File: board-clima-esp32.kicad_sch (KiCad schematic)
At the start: 54 parts, among them IC1 ESP32-S3-WROOM-1-N4, J1 Conn_01x06_Pin, J2 Screw_Terminal_01x03, J3 Conn_01x04_Pin, J5 Conn_01x05_Pin, J6 USB_C_Receptacle, Q1 AO3400A, Q2 AO3401A, Q3 AO3400A, SW1 RESET, SW2 BOOT, U1 AMS1117-3.3, U3 PC817, U4 PC817

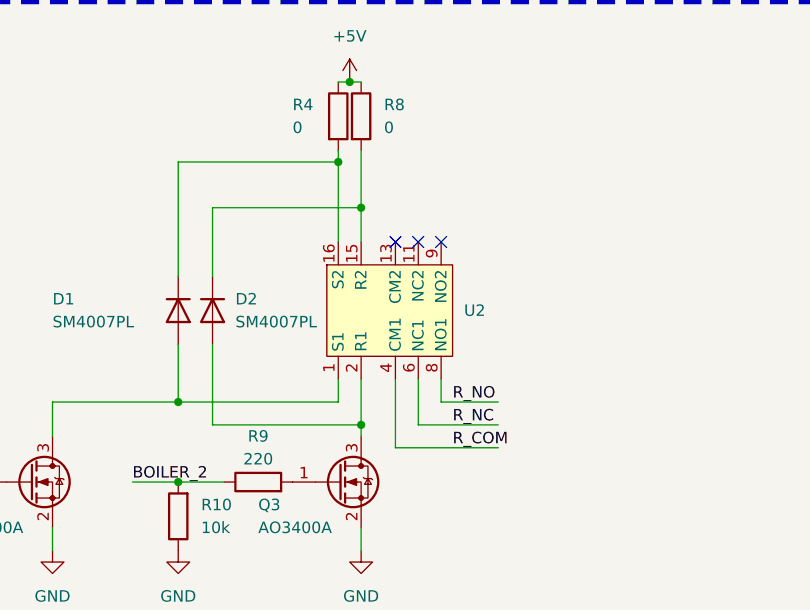
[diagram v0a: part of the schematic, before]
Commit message: rev2 routing
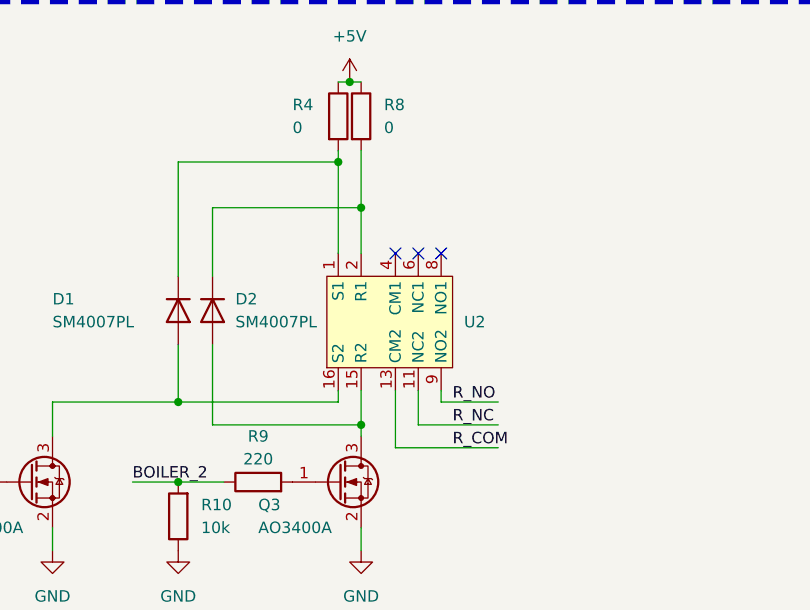
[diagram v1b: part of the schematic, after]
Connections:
- net R_COM: now also U2.13 (CM2); no longer U2.4 (CM1)
- net R_NC: now also U2.11 (NC2); no longer U2.6 (NC1)
- net R_NO: now also U2.9 (NO2); no longer U2.8 (NO1)
- net at D1.2 (A), Q1.3 (D): now also U2.16 (S2); no longer U2.1 (S1)
- net at D2.1 (K), R8.2: now also U2.2 (R1); no longer U2.15 (R2)
- net at D1.1 (K), R4.2: now also U2.1 (S1); no longer U2.16 (S2)
- net at D2.2 (A), Q3.3 (D): now also U2.15 (R2); no longer U2.2 (R1)
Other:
- moved on the sheet: U2
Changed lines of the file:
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@@
   (junction (at 240.03 72.39) (diameter 0) (color 0 0 0 0)
   )
+  (junction (at 198.12 135.89) (diameter 0) (color 0 0 0 0)
+  )
+  (junction (at 102.87 26.67) (diameter 0) (color 0 0 0 0)
+  )
+  (junction (at 209.55 120.65) (diameter 0) (color 0 0 0 0)
+  )
+  (junction (at 300.99 78.74) (diameter 0) (color 0 0 0 0)
+  )
+  (junction (at 93.98 26.67) (diameter 0) (color 0 0 0 0)
+  )
+  (junction (at 240.03 69.85) (diameter 0) (color 0 0 0 0)
+  )
+  (junction (at 182.88 34.29) (diameter 0) (color 0 0 0 0)
+  )
+  (junction (at 182.88 85.09) (diameter 0) (color 0 0 0 0)
+  )
+  (junction (at 115.57 39.37) (diameter 0) (color 0 0 0 0)
+  )
+  (junction (at 186.69 99.06) (diameter 0) (color 0 0 0 0)
+  )
   (junction (at 92.71 152.4) (diameter 0) (color 0 0 0 0)
-  )
-  (junction (at 198.12 135.89) (diameter 0) (color 0 0 0 0)
-  )
-  (junction (at 102.87 26.67) (diameter 0) (color 0 0 0 0)
-  )
-  (junction (at 209.55 120.65) (diameter 0) (color 0 0 0 0)
-  )
-  (junction (at 300.99 78.74) (diameter 0) (color 0 0 0 0)
-  )
-  (junction (at 93.98 26.67) (diameter 0) (color 0 0 0 0)
-  )
-  (junction (at 240.03 69.85) (diameter 0) (color 0 0 0 0)
-  )
-  (junction (at 182.88 34.29) (diameter 0) (color 0 0 0 0)
-  )
-  (junction (at 182.88 85.09) (diameter 0) (color 0 0 0 0)
-  )
-  (junction (at 115.57 39.37) (diameter 0) (color 0 0 0 0)
-  )
-  (junction (at 186.69 99.06) (diameter 0) (color 0 0 0 0)
   )
   (junction (at 198.12 146.05) (diameter 0) (color 0 0 0 0)
@@
   (no_connect (at 240.03 52.07))
   (no_connect (at 45.72 64.77))
-  (no_connect (at 101.6 132.08))
   (no_connect (at 45.72 59.69))
   (no_connect (at 240.03 46.99))
@@
   (no_connect (at 45.72 57.15))
   (no_connect (at 207.01 44.45))
+  (no_connect (at 101.6 133.35))
   (no_connect (at 45.72 49.53))
   (no_connect (at 45.72 72.39))
@@
   (no_connect (at 45.72 82.55))
   (no_connect (at 240.03 34.29))
-  (no_connect (at 99.06 132.08))
   (no_connect (at 240.03 44.45))
   (no_connect (at 45.72 67.31))
@@
   (no_connect (at 45.72 74.93))
   (no_connect (at 207.01 67.31))
-  (no_connect (at 96.52 132.08))
+  (no_connect (at 99.06 133.35))
   (no_connect (at 207.01 49.53))
   (no_connect (at 207.01 54.61))
@@
   (no_connect (at 207.01 36.83))
   (no_connect (at 45.72 52.07))
+  (no_connect (at 96.52 133.35))
   (no_connect (at 207.01 57.15))
   (no_connect (at 240.03 36.83))
@@
     (stroke (width 0) (type default))
   )
+  (wire (pts (xy 92.71 148.59) (xy 92.71 152.4))
+    (stroke (width 0) (type default))
+  )
   (wire (pts (xy 397.51 77.47) (xy 403.86 77.47))
     (stroke (width 0) (type default))
@@
     (stroke (width 0) (type default))
   )
+  (wire (pts (xy 90.17 123.19) (xy 90.17 133.35))
+    (stroke (width 0) (type default))
+  )
   (wire (pts (xy 189.23 99.06) (xy 186.69 99.06))
     (stroke (width 0) (type default))
@@
     (stroke (width 0) (type default))
   )
-  (wire (pts (xy 90.17 147.32) (xy 90.17 149.86))
-    (stroke (width 0) (type default))
-  )
   (wire (pts (xy 45.72 24.13) (xy 53.34 24.13))
     (stroke (width 0) (type default))
@@
     (stroke (width 0) (type default))
   )
-  (wire (pts (xy 90.17 123.19) (xy 90.17 132.08))
-    (stroke (width 0) (type default))
-  )
   (wire (pts (xy 160.02 34.29) (xy 168.91 34.29))
     (stroke (width 0) (type default))
@@
     (stroke (width 0) (type default))
   )
+  (wire (pts (xy 92.71 128.27) (xy 92.71 133.35))
+    (stroke (width 0) (type default))
+  )
   (wire (pts (xy 300.99 73.66) (xy 300.99 78.74))
     (stroke (width 0) (type default))
@@
     (stroke (width 0) (type default))
   )
-  (wire (pts (xy 96.52 147.32) (xy 96.52 154.94))
-    (stroke (width 0) (type default))
-  )
   (wire (pts (xy 195.58 59.69) (xy 207.01 59.69))
     (stroke (width 0) (type default))
@@
     (stroke (width 0) (type default))
   )
+  (wire (pts (xy 99.06 148.59) (xy 99.06 152.4))
+    (stroke (width 0) (type default))
+  )
   (wire (pts (xy 209.55 128.27) (xy 209.55 130.81))
     (stroke (width 0) (type default))
@@
     (stroke (width 0) (type default))
   )
-  (wire (pts (xy 92.71 147.32) (xy 92.71 152.4))
-    (stroke (width 0) (type default))
-  )
   (wire (pts (xy 102.87 36.83) (xy 102.87 39.37))
     (stroke (width 0) (type default))
@@
     (stroke (width 0) (type default))
   )
+  (wire (pts (xy 96.52 148.59) (xy 96.52 154.94))
+    (stroke (width 0) (type default))
+  )
   (wire (pts (xy 173.99 128.27) (xy 173.99 130.81))
     (stroke (width 0) (type default))
@@
     (stroke (width 0) (type default))
   )
-  (wire (pts (xy 99.06 147.32) (xy 99.06 152.4))
-    (stroke (width 0) (type default))
-  )
   (wire (pts (xy 128.27 26.67) (xy 134.62 26.67))
     (stroke (width 0) (type default))
@@
     (stroke (width 0) (type default))
   )
+  (wire (pts (xy 90.17 148.59) (xy 90.17 149.86))
+    (stroke (width 0) (type default))
+  )
   (wire (pts (xy 166.37 140.97) (xy 173.99 140.97))
     (stroke (width 0) (type default))
   )
-  (wire (pts (xy 101.6 147.32) (xy 101.6 149.86))
-    (stroke (width 0) (type default))
-  )
   (wire (pts (xy 96.52 154.94) (xy 107.95 154.94))
     (stroke (width 0) (type default))
   )
+  (wire (pts (xy 101.6 148.59) (xy 101.6 149.86))
+    (stroke (width 0) (type default))
+  )
   (wire (pts (xy 198.12 133.35) (xy 198.12 135.89))
     (stroke (width 0) (type default))
@@
   )
   (wire (pts (xy 299.72 76.2) (xy 302.26 76.2))
-    (stroke (width 0) (type default))
-  )
-  (wire (pts (xy 92.71 128.27) (xy 92.71 132.08))
     (stroke (width 0) (type default))
   )
@@
     )
   )
-  (symbol (lib_id "HFD2:HFD2/00X-M-L2") (at 88.9 134.62 0) (unit 1)
-    (in_bom yes) (on_board yes) (dnp no) (fields_autoplaced)
-    (property "Reference" "U2" (at 104.14 139.7 0)
+  (symbol (lib_id "HFD2:HFD2/00X-M-L2") (at 88.9 146.05 0) (mirror x) (unit 1)
+    (in_bom yes) (on_board yes) (dnp no)
+    (property "Reference" "U2" (at 104.14 140.97 0)
       (effects (font (size 1.27 1.27)) (justify left))
     )
-    (property "Value" "~" (at 88.9 134.62 0)
+    (property "Value" "~" (at 88.9 146.05 0)
       (effects (font (size 1.27 1.27)))
     )
-    (property "Footprint" "HFD2:HFD2-00X-M-L2" (at 96.52 120.65 0)
-      (effects (font (size 1.27 1.27)) hide)
-    )
-    (property "Datasheet" "https://pdf1.alldatasheet.com/datasheet-pdf/download/660910/HONGFA/HFD2SLASH005-S-L2-D.html" (at 93.98 123.19 0)
-      (effects (font (size 1.27 1.27)) hide)
-    )
+    (property "Footprint" "HFD2:HFD2-00X-M-L2" (at 96.52 160.02 0)
+      (effects (font (size 1.27 1.27)) hide)
+    )
+    (property "Datasheet" "https://pdf1.alldatasheet.com/datasheet-pdf/download/660910/HONGFA/HFD2SLASH005-S-L2-D.html" (at 93.98 157.48 0)
+      (effects (font (size 1.27 1.27)) hide)
+    )
